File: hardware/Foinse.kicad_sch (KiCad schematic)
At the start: 150 parts, among them J1 Conn_02x03_Odd_Even, J10 Conn_02x03_Odd_Even, J2 2060-1452, J3 ESQ-110-14-G-D, J4 PJ-002AH, J5 2060-1452/998-404, J8 2601-1108, J9 USB_C_Receptacle_USB2.0_16P, Q1 AO3400A, Q10 AO3400A, Q11 AO3400A, Q12 AO3400A, Q13 AO3400A, Q14 AO3400A, Q2 AO3400A, Q3 AO3400A, Q4 AO3400A, Q5 AO3400A, Q6 AO3400A, Q7 AO3400A, Q8 AO3400A, Q9 AO3400A, U1 STM32F072C8Tx, U10 LTV-817, U11 LTV-817, U12 LTV-817, U13 LTV-817, U14 USBLC6-2SC6, U15 INA239AIDGSR, U16 INA239AIDGSR, U17 LTC4412xS6, U18 LTV-817, U19 TPS56A37RPAR, U2 TLV70433DBVT, U3 LTV-817, U4 TJA1051T-3, U5 TPS563203, U7 LTV-817, U8 LTV-817, U9 LTV-817

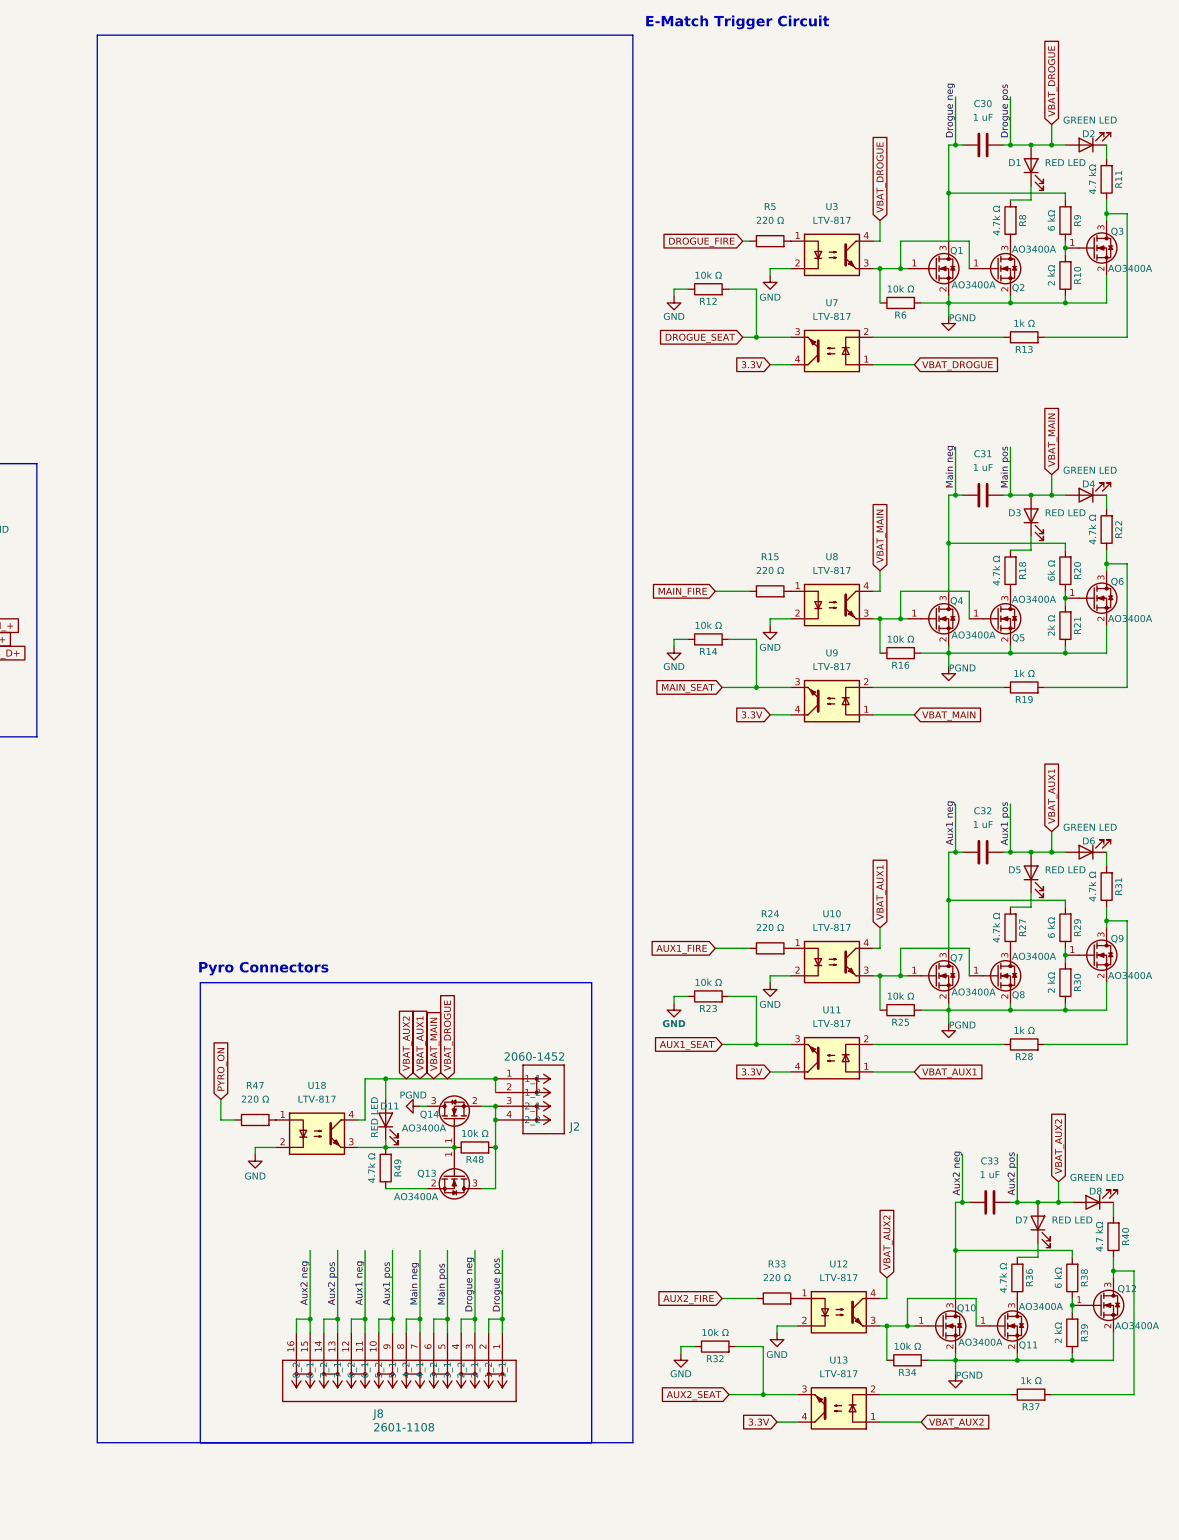
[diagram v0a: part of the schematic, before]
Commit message: folders are indded cool
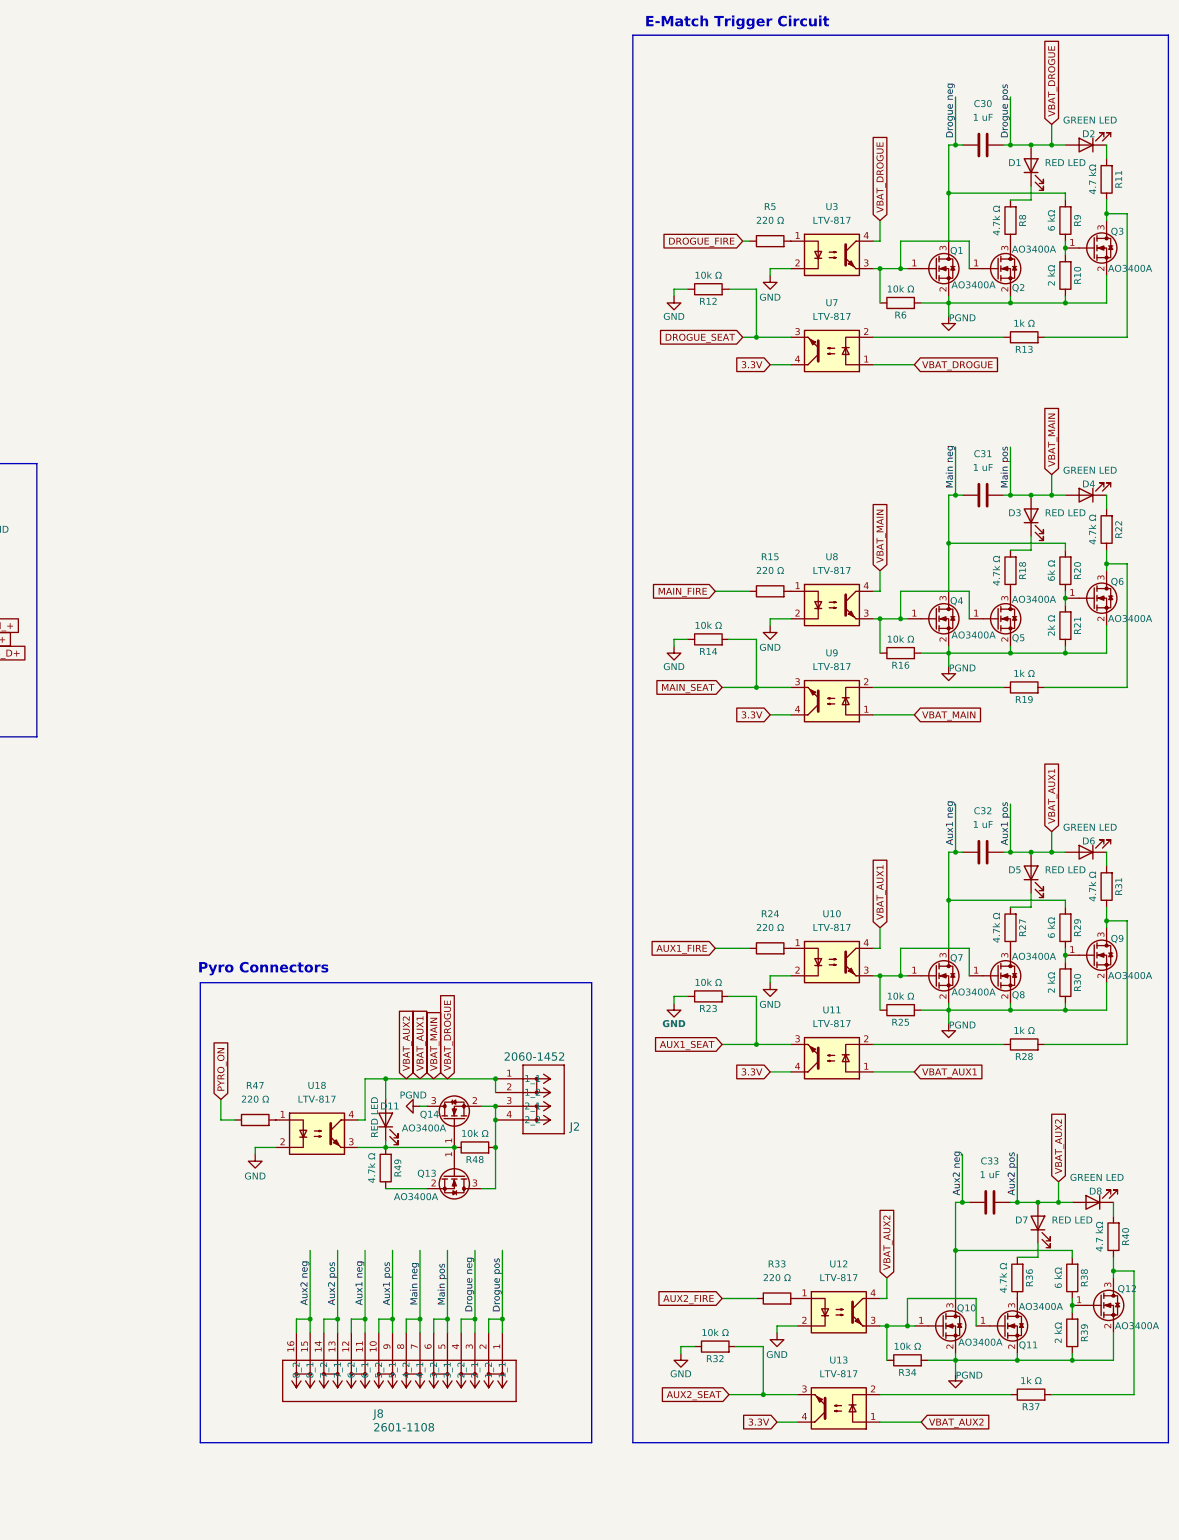
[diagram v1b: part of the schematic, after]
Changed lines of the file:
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@@
 		(exclude_from_sim no)
 		(at 476.25 21.59 0)
-		(size -99.06 260.35)
+		(size 99.06 260.35)
 		(margins 0.9525 0.9525 0.9525 0.9525)
 		(stroke

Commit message: minor changes
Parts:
- removed C30, C31, C33: 1 uF, Capacitor_SMD:C_0402_1005Metric, symbol Device:C
- removed D1, D11, D3, D5, D7: RED LED, LED_SMD:LED_0402_1005Metric, symbol Device:LED
- removed D2, D4, D6, D8: GREEN LED, LED_SMD:LED_0402_1005Metric, symbol Device:LED
- removed J1, J10: Conn_02x03_Odd_Even, Connector_PinHeader_1.00mm:PinHeader_2x03_P1.00mm_Vertical, symbol Connector_Generic:Conn_02x03_Odd_Even
- removed J2: 2060-1452, Foinse Footprints:WAG, symbol Wago_2060-1452 998-404:2060-1452_998-404
- removed J3: ESQ-110-14-G-D, Foinse Footprints:SAMTEC_ESQ-110-14-G-D, symbol ESQ-110-X-X-D:ESQ-110-X-X-D
- removed J5: 2060-1452/998-404, Foinse Footprints:WAG, symbol Wago_2060-1452 998-404:2060-1452_998-404
- removed J8: 2601-1108, Foinse Footprints:CONN8_2601-1108_WAG, symbol Wago_2601-1104:2601-1108
- removed J9: USB_C_Receptacle_USB2.0_16P, Connector_USB:USB_C_Receptacle_G-Switch_GT-USB-7010ASV, symbol Connector:USB_C_Receptacle_USB2.0_16P
- removed Q1, Q10, Q11, Q12, Q13, Q14, Q2, Q3, Q4, Q5, Q6, Q7, Q8, Q9: AO3400A, Package_TO_SOT_SMD:SOT-23, symbol Transistor_FET:AO3400A
- removed R10, R30, R39: 2 kΩ, Resistor_SMD:R_0402_1005Metric, symbol Device:R
- removed R11, R40: 4.7 kΩ, Resistor_SMD:R_0402_1005Metric, symbol Device:R
- removed R12, R14, R16, R23, R25, R32, R34, R48, R6: 10k Ω, Resistor_SMD:R_0402_1005Metric, symbol Device:R
- removed R13, R19, R28, R37: 1k Ω, Resistor_SMD:R_0402_1005Metric, symbol Device:R
- removed R15, R24, R33, R47: 220 Ω, Resistor_SMD:R_0402_1005Metric, symbol Device:R
- removed R18, R22, R27, R31, R36, R49, R8: 4.7k Ω, Resistor_SMD:R_0402_1005Metric, symbol Device:R
- removed R20: 6k Ω, Resistor_SMD:R_0402_1005Metric, symbol Device:R
- removed R21: 2k Ω, Resistor_SMD:R_0402_1005Metric, symbol Device:R
- removed R29, R38, R9: 6 kΩ, Resistor_SMD:R_0402_1005Metric, symbol Device:R
- removed R41, R42: 5.1K, Resistor_SMD:R_0402_1005Metric, symbol Device:R
- removed R43, R44: 10K, Resistor_SMD:R_0402_1005Metric, symbol Device:R
- removed U10, U11, U12, U13, U18, U3, U7, U8, U9: LTV-817, Foinse Footprints:SO4_TOS, symbol Isolator:LTV-817
- removed U14: USBLC6-2SC6, Package_TO_SOT_SMD:SOT-23-6, symbol Power_Protection:USBLC6-2SC6
- added J1: ESQ-110-X-X-D, SAMTEC_ESQ-110-14-G-D, symbol ESQ-110-X-X-D:ESQ-110-X-X-D
- added J2: XT30PW-M, footprints:AMASS_XT30PW-M, symbol XT30PW-M:XT30PW-M
- added J6: JTAG-10 PIN, Connector_IDC:IDC-Header_2x05_P2.54mm_Vertical, symbol Connector_Generic_MountingPin:Conn_01x10_MountingPin
- C32: value 1 uF -> 100nF
- R5: value 220 Ω -> 10kΩ
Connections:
- net Aux1 neg is gone; now on net GND: C32.2
- net VBAT_AUX1 is gone; now on net NRST: C32.1
- net 3.3V: now also J6.7 (Pin_7), J6.8 (Pin_8)
- net GND: now also R5.2, J1.03, J1.04, J1.07, J1.08, J1.14, J1.19, J1.20, J2.N, J6.5 (Pin_5), J6.6 (Pin_6)
- net NRST: now also J1.17, J6.1 (Pin_1)
- net SWDIO: now also J1.15, J6.4 (Pin_4)
- net at MOSFET1.2 (D), U17.1 (VIN): now also J2.P
- net at U1.44 (BOOT0): now also R5.1
- net AUX1_FIRE: no longer names the net of U1.41 (PB5)
- net AUX1_SEAT: no longer names the net of U1.25 (PB12)
- net AUX2_FIRE: no longer names the net of U1.42 (PB6)
- net AUX2_SEAT: no longer names the net of U1.26 (PB13)
- net DROGUE_FIRE: no longer names the net of U1.39 (PB3)
- net DROGUE_FIRE: no longer R5.1
- net DROGUE_SEAT: no longer names the net of U1.21 (PB10)
- net MAIN_FIRE: no longer names the net of U1.40 (PB4)
- net MAIN_SEAT: no longer names the net of U1.22 (PB11)
- net Mode_sel: no longer names the net of U1.45 (PB8)
- net PYRO_ON: no longer names the net of U1.43 (PB7)
- net SWCLK renamed SWCLK3
- net SWCLK3: now also J1.11, J6.2 (Pin_2)
- new net 5V_LOGIC: J1.05, J1.06
- new net 5v_SERVO: J1.01, J1.02
- new net CAN_o+: J1.16
- new net CAN_o-: J1.18
- no-connect marks 6 -> 12
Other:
- note added: "Connector_IDC:IDC-Header_2x05_P2.54mm_Vertical"
- note added: "what is the current and voltage rating for this?"
- note removed: "E-Match Trigger Circuit"
- note removed: "Pyro Connectors"
- note removed: "USB-C"
- note removed: "USB-C & mode select"
- moved on the sheet: C1, C10, C11, C12, C13, C14, C15, C16, C17, C18, C19, C2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
